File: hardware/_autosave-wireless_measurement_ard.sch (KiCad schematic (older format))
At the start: 25 parts, among them J1 Conn_01x08, SW1 SW_SPDT, U1 EFM8LB1, U2 JDY-08, U3 MCP16415, U4 MAX44284

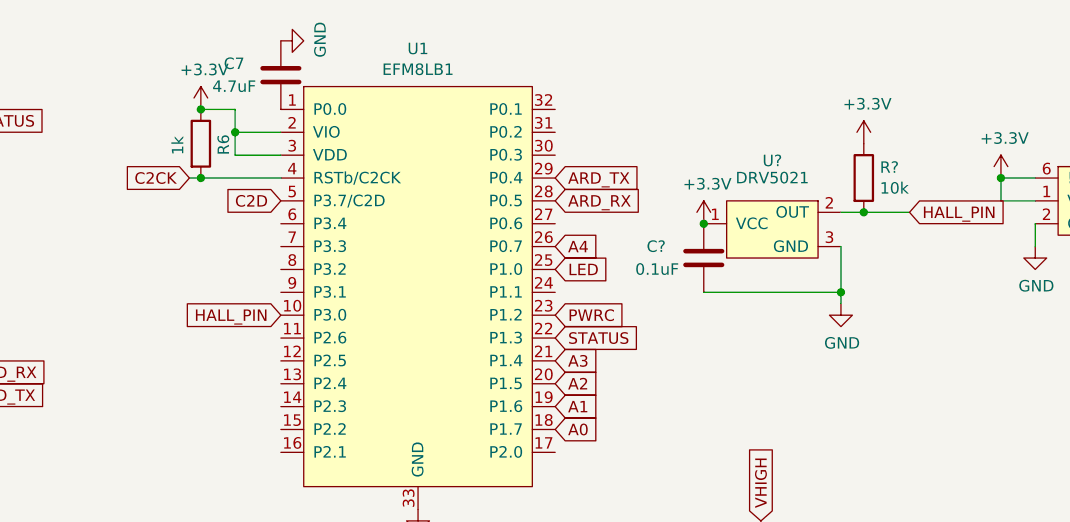
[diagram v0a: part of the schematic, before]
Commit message: Added new code for mini
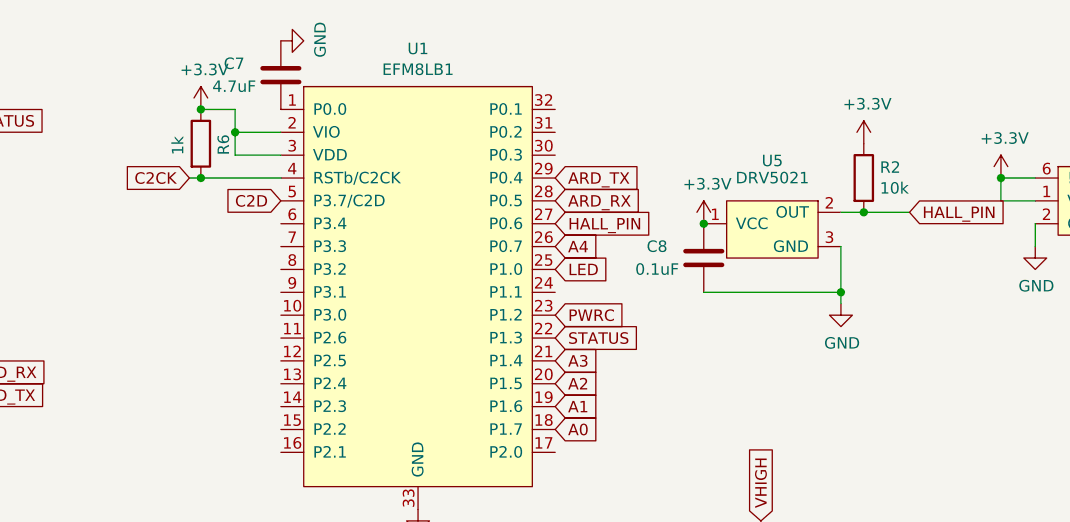
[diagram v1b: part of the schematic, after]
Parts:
- gave numbers to parts that had none: 3
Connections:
- net HALL_PIN: now also U1.27 (P0.6); no longer U1.10 (P3.0)
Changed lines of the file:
@@
 	0    -1   -1   0
 $EndComp
-Text GLabel 5250 2150 0    50   Input ~ 0
+Text GLabel 6450 1750 2    50   Input ~ 0
 HALL_PIN
 $Comp
-L ben_common:DRV5021 U?
+L ben_common:DRV5021 U5
 U 1 1 6148F942
 P 7400 1750
-F 0 "U?" H 7400 2025 50  0000 C CNN
+F 0 "U5" H 7400 2025 50  0000 C CNN
 F 1 "DRV5021" H 7400 1950 50  0000 C CNN
 F 2 "Package_TO_SOT_SMD:SOT-23" H 7100 1950 50  0001 C CNN
@@
 $EndComp
 $Comp
-L power:GND #PWR?
+L power:GND #PWR0105
 U 1 1 6149026D
 P 7700 2100
-F 0 "#PWR?" H 7700 1850 50  0001 C CNN
+F 0 "#PWR0105" H 7700 1850 50  0001 C CNN
 F 1 "GND" H 7705 1927 50  0000 C CNN
 F 2 "" H 7700 2100 50  0001 C CNN
@@
 $EndComp
 $Comp
-L power:+3.3V #PWR?
+L power:+3.3V #PWR0117
 U 1 1 61490741
 P 7100 1750
-F 0 "#PWR?" H 7100 1600 50  0001 C CNN
+F 0 "#PWR0117" H 7100 1600 50  0001 C CNN
 F 1 "+3.3V" H 7115 1923 50  0000 C CNN
 F 2 "" H 7100 1750 50  0001 C CNN
@@
 $EndComp
 $Comp
-L power:+3.3V #PWR?
+L power:+3.3V #PWR0120
 U 1 1 61490CF5
 P 7800 1400
-F 0 "#PWR?" H 7800 1250 50  0001 C CNN
+F 0 "#PWR0120" H 7800 1250 50  0001 C CNN
 F 1 "+3.3V" H 7815 1573 50  0000 C CNN
 F 2 "" H 7800 1400 50  0001 C CNN
@@
 $EndComp
 $Comp
-L Device:R R?
+L Device:R R2
 U 1 1 614912CF
 P 7800 1550
-F 0 "R?" H 7870 1596 50  0000 L CNN
+F 0 "R2" H 7870 1596 50  0000 L CNN
 F 1 "10k" H 7870 1505 50  0000 L CNN
 F 2 "Resistor_SMD:R_0603_1608Metric_Pad0.98x0.95mm_HandSolder" V 7730 1550 50  0001 C CNN
@@
 Connection ~ 7800 1700
 $Comp
-L Device:C C?
+L Device:C C8
 U 1 1 6149AFDF
 P 7100 1900
-F 0 "C?" H 6850 1950 50  0000 L CNN
+F 0 "C8" H 6850 1950 50  0000 L CNN
 F 1 "0.1uF" H 6800 1850 50  0000 L CNN
 F 2 "Capacitor_SMD:C_0603_1608Metric_Pad1.08x0.95mm_HandSolder" H 7138 1750 50  0001 C CNN
